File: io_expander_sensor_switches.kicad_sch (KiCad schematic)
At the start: 8 parts

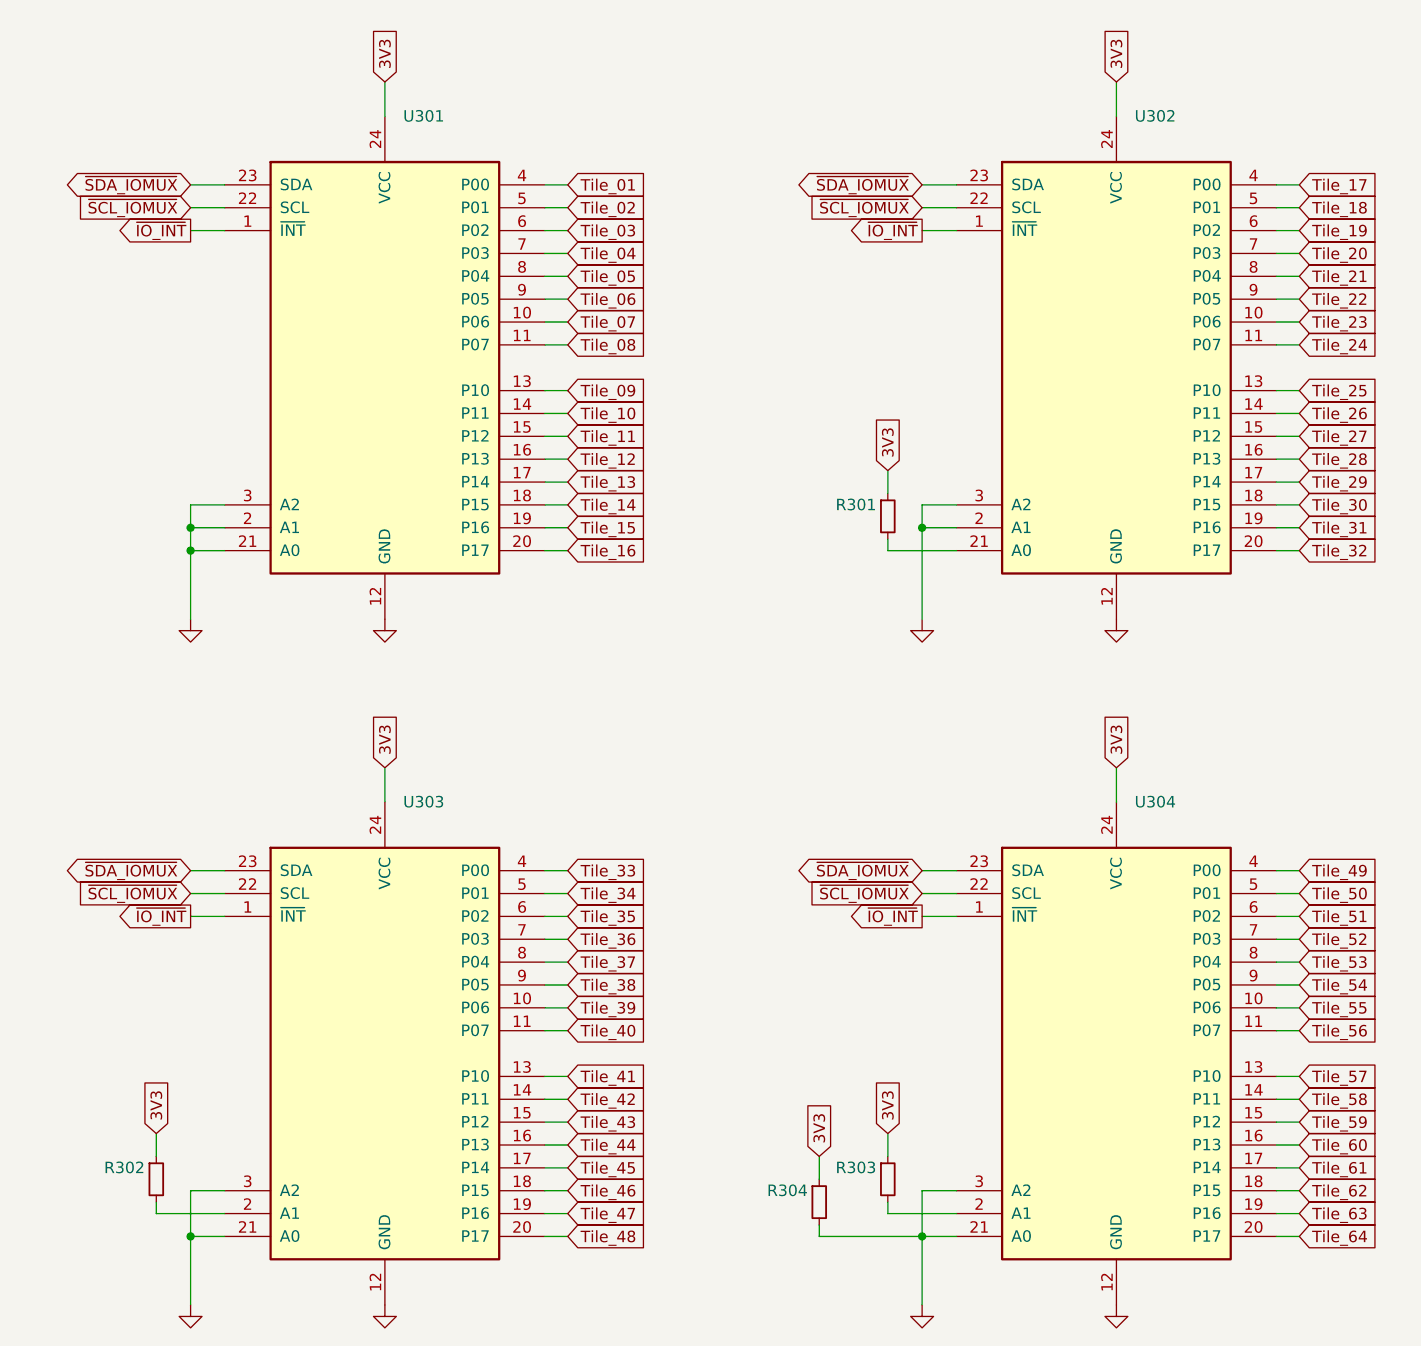
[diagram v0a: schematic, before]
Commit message: refactor IO expander pin assignment
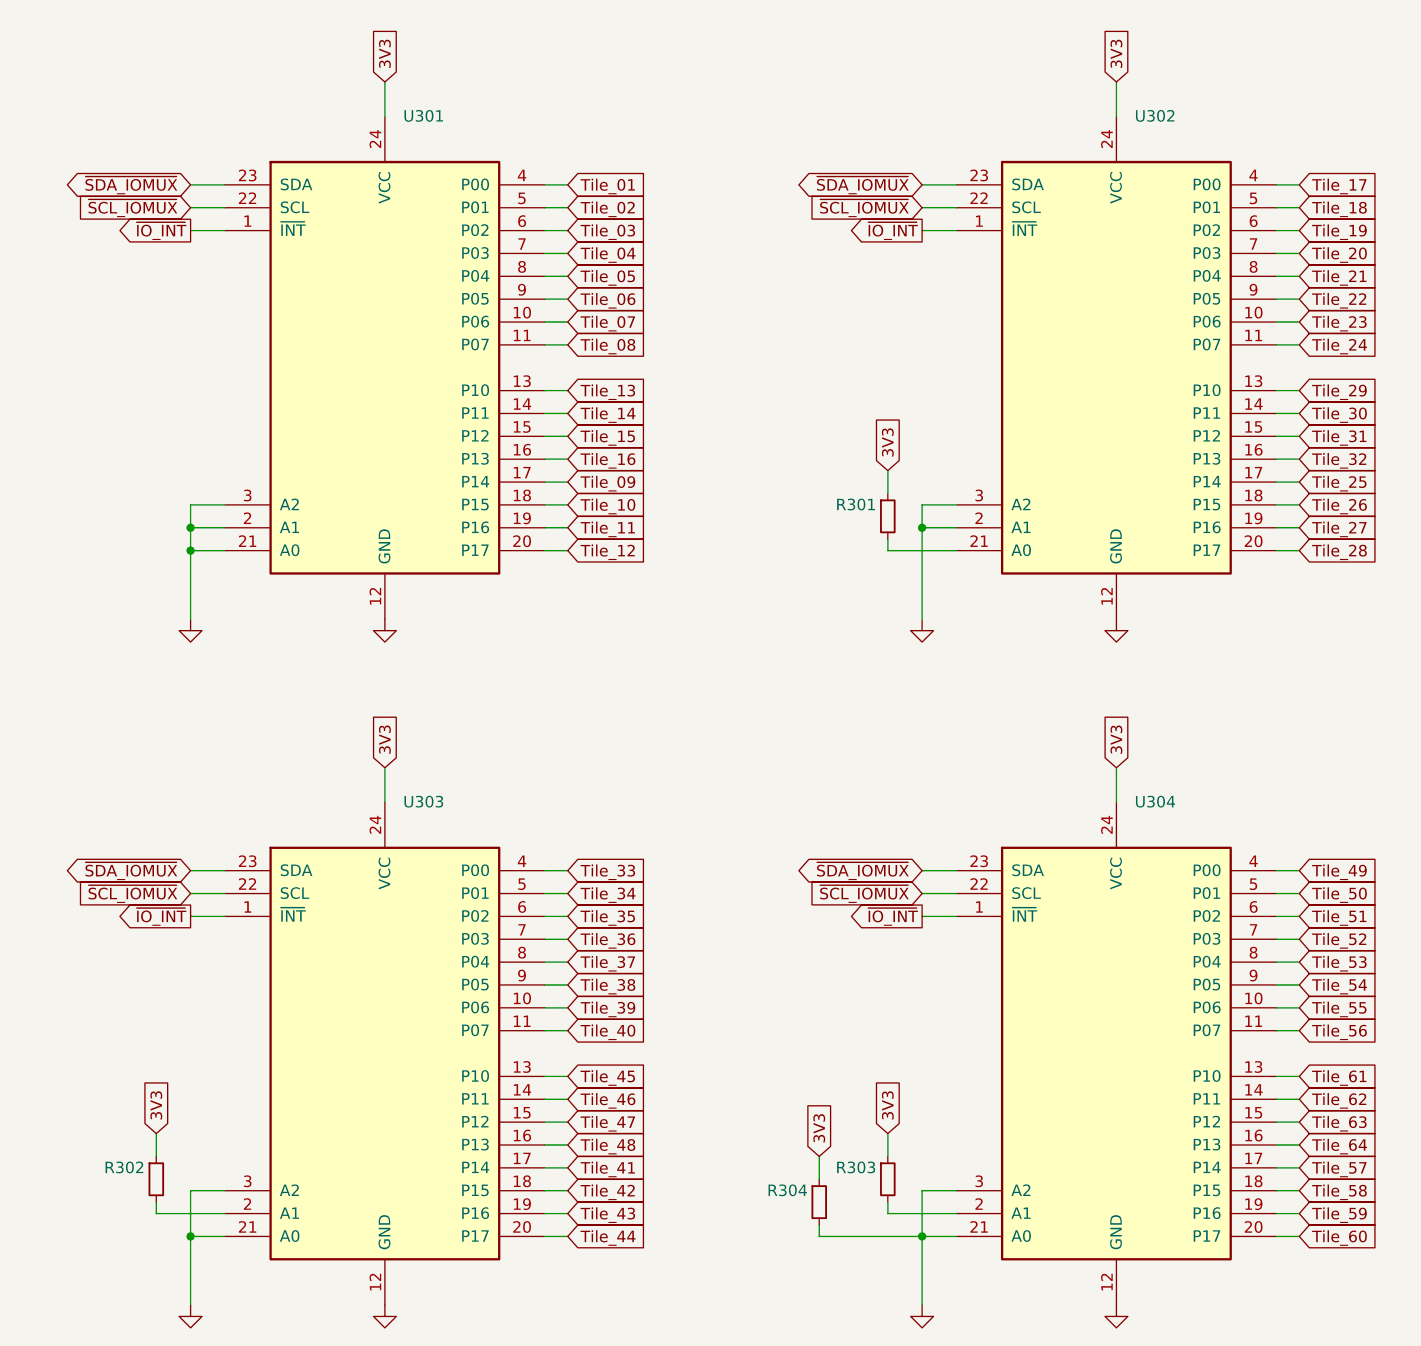
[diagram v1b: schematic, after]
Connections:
- net Tile_09: now also U301.17 (P14); no longer U301.13 (P10)
- net Tile_10: now also U301.18 (P15); no longer U301.14 (P11)
- net Tile_11: now also U301.19 (P16); no longer U301.15 (P12)
- net Tile_12: now also U301.20 (P17); no longer U301.16 (P13)
- net Tile_13: now also U301.13 (P10); no longer U301.17 (P14)
- net Tile_14: now also U301.14 (P11); no longer U301.18 (P15)
- net Tile_15: now also U301.15 (P12); no longer U301.19 (P16)
- net Tile_16: now also U301.16 (P13); no longer U301.20 (P17)
- net Tile_25: now also U302.17 (P14); no longer U302.13 (P10)
- net Tile_26: now also U302.18 (P15); no longer U302.14 (P11)
- net Tile_27: now also U302.19 (P16); no longer U302.15 (P12)
- net Tile_28: now also U302.20 (P17); no longer U302.16 (P13)
- net Tile_29: now also U302.13 (P10); no longer U302.17 (P14)
- net Tile_30: now also U302.14 (P11); no longer U302.18 (P15)
- net Tile_31: now also U302.15 (P12); no longer U302.19 (P16)
- net Tile_32: now also U302.16 (P13); no longer U302.20 (P17)
- net Tile_41: now also U303.17 (P14); no longer U303.13 (P10)
- net Tile_42: now also U303.18 (P15); no longer U303.14 (P11)
- net Tile_43: now also U303.19 (P16); no longer U303.15 (P12)
- net Tile_44: now also U303.20 (P17); no longer U303.16 (P13)
- net Tile_45: now also U303.13 (P10); no longer U303.17 (P14)
- net Tile_46: now also U303.14 (P11); no longer U303.18 (P15)
- net Tile_47: now also U303.15 (P12); no longer U303.19 (P16)
- net Tile_48: now also U303.16 (P13); no longer U303.20 (P17)
- net Tile_57: now also U304.17 (P14); no longer U304.13 (P10)
- net Tile_58: now also U304.18 (P15); no longer U304.14 (P11)
- net Tile_59: now also U304.19 (P16); no longer U304.15 (P12)
- net Tile_60: now also U304.20 (P17); no longer U304.16 (P13)
- net Tile_61: now also U304.13 (P10); no longer U304.17 (P14)
- net Tile_62: now also U304.14 (P11); no longer U304.18 (P15)
- net Tile_63: now also U304.15 (P12); no longer U304.19 (P16)
- net Tile_64: now also U304.16 (P13); no longer U304.20 (P17)
